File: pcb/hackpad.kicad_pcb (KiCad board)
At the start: 2 copper layers, 21.5 x 50 mm, 4 parts, among them SW1 SW_Push, SW2 SW_Push, SW3 SW_Push, U1 MOUDLE-SEEEDUINO-XIAO

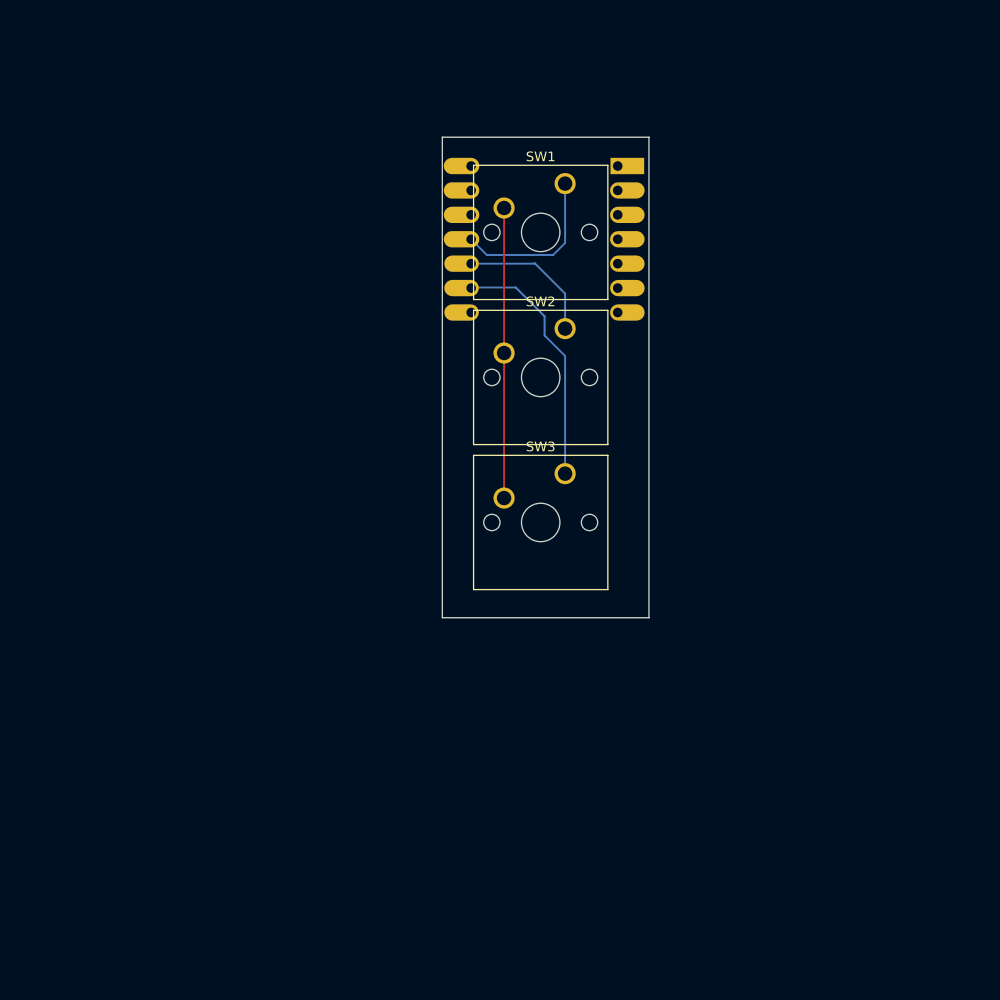
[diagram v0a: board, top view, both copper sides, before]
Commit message: Update the schematic
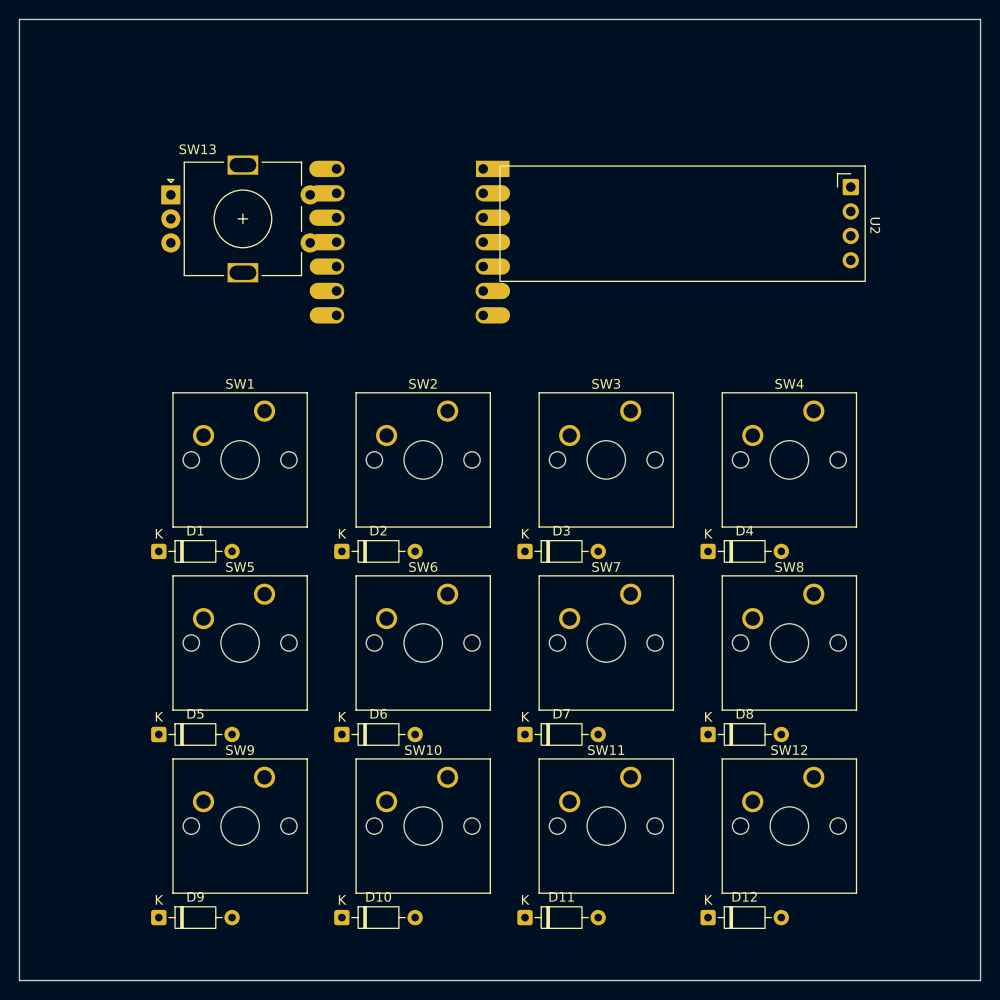
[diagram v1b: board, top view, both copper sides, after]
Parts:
- added D1: 1N4148, Diode_THT:D_DO-35_SOD27_P7.62mm_Horizontal, F.Cu at (49.0, 84.6)
- added D10: 1N4148, Diode_THT:D_DO-35_SOD27_P7.62mm_Horizontal, F.Cu at (68.0, 122.7)
- added D11: 1N4148, Diode_THT:D_DO-35_SOD27_P7.62mm_Horizontal, F.Cu at (87.1, 122.7)
- added D12: 1N4148, Diode_THT:D_DO-35_SOD27_P7.62mm_Horizontal, F.Cu at (106.2, 122.7)
- added D2: 1N4148, Diode_THT:D_DO-35_SOD27_P7.62mm_Horizontal, F.Cu at (68.0, 84.6)
- added D3: 1N4148, Diode_THT:D_DO-35_SOD27_P7.62mm_Horizontal, F.Cu at (87.1, 84.6)
- added D4: 1N4148, Diode_THT:D_DO-35_SOD27_P7.62mm_Horizontal, F.Cu at (106.2, 84.6)
- added D5: 1N4148, Diode_THT:D_DO-35_SOD27_P7.62mm_Horizontal, F.Cu at (49.0, 103.7)
- added D6: 1N4148, Diode_THT:D_DO-35_SOD27_P7.62mm_Horizontal, F.Cu at (68.0, 103.7)
- added D7: 1N4148, Diode_THT:D_DO-35_SOD27_P7.62mm_Horizontal, F.Cu at (87.1, 103.7)
- added D8: 1N4148, Diode_THT:D_DO-35_SOD27_P7.62mm_Horizontal, F.Cu at (106.2, 103.7)
- added D9: 1N4148, Diode_THT:D_DO-35_SOD27_P7.62mm_Horizontal, F.Cu at (49.0, 122.7)
- added SW10: SW_Push, Button_Switch_Keyboard:SW_Cherry_MX_1.00u_PCB, F.Cu at (79.0, 108.1)
- added SW11: SW_Push, Button_Switch_Keyboard:SW_Cherry_MX_1.00u_PCB, F.Cu at (98.1, 108.1)
- added SW12: SW_Push, Button_Switch_Keyboard:SW_Cherry_MX_1.00u_PCB, F.Cu at (117.2, 108.1)
- added SW13: RotaryEncoder_Switch, Rotary_Encoder:RotaryEncoder_Alps_EC11E-Switch_Vertical_H20mm, F.Cu at (50.2, 47.5)
- added SW4: SW_Push, Button_Switch_Keyboard:SW_Cherry_MX_1.00u_PCB, F.Cu at (117.2, 70.0)
- added SW5: SW_Push, Button_Switch_Keyboard:SW_Cherry_MX_1.00u_PCB, F.Cu at (60.0, 89.0)
- added SW6: SW_Push, Button_Switch_Keyboard:SW_Cherry_MX_1.00u_PCB, F.Cu at (79.0, 89.0)
- added SW7: SW_Push, Button_Switch_Keyboard:SW_Cherry_MX_1.00u_PCB, F.Cu at (98.1, 89.0)
- added SW8: SW_Push, Button_Switch_Keyboard:SW_Cherry_MX_1.00u_PCB, F.Cu at (117.2, 89.0)
- added SW9: SW_Push, Button_Switch_Keyboard:SW_Cherry_MX_1.00u_PCB, F.Cu at (60.0, 108.1)
- added U2: ER_OLEDM0.91_1x-I2C, Display:ER_OLEDM0.91_1x-I2C, F.Cu at (121.0, 46.7)
- moved SW1 39.2 mm to (60.0, 70.0)
- moved SW2 14.9 mm to (79.0, 70.0)
- moved U1 14.0 mm to (75.1, 52.4)
- moved SW3 9.43 mm to (98.1, 70.0)
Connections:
- SW1 pad 1: Net-(U1-PA6_A10_D10_MOSI) -> /Column 0
- SW1 pad 2: GND -> Net-(D1-A)
- SW2 pad 1: Net-(U1-PA5_A9_D9_MISO) -> /Column 1
- SW2 pad 2: GND -> Net-(D2-A)
- SW3 pad 1: Net-(U1-PA7_A8_D8_SCK) -> /Column 2
- SW3 pad 2: GND -> Net-(D3-A)
- U1 pad 1: unconnected-(U1-PA02_A0_D0-Pad1) -> /Column 0
- U1 pad 12: unconnected-(U1-3V3-Pad12) -> Net-(U1-3V3)
- U1 pad 2: unconnected-(U1-PA4_A1_D1-Pad2) -> /Column 1
- U1 pad 3: unconnected-(U1-PA10_A2_D2-Pad3) -> /Column 2
- U1 pad 4: unconnected-(U1-PA11_A3_D3-Pad4) -> /Column 3
- U1 pad 5: unconnected-(U1-PA8_A4_D4_SDA-Pad5) -> OLED SDA
- U1 pad 6: unconnected-(U1-PA9_A5_D5_SCL-Pad6) -> OLED SCL
- U1 pad 7: unconnected-(U1-PB08_A6_D6_TX-Pad7) -> Net-(D1-K)
- U1 pad 8: unconnected-(U1-PB09_A7_D7_RX-Pad8) -> /Row 1
- U1 pad 9: Net-(U1-PA7_A8_D8_SCK) -> /Row 2
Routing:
- net GND: track 30.2 -> 0.00 mm
- net Net-(U1-PA7_A8_D8_SCK): track 26.2 -> 0.00 mm
- net Net-(U1-PA6_A10_D10_MOSI): track 17.2 -> 0.00 mm
- net Net-(U1-PA5_A9_D9_MISO): track 14.7 -> 0.00 mm
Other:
- board size 21.5 x 50 mm -> 100 x 100 mm
